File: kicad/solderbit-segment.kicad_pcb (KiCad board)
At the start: 2 copper layers, 25 x 50 mm, 15 parts, among them J1 Conn_01x05_Pin, U1 PCF8574AT, U2 PCF8574N

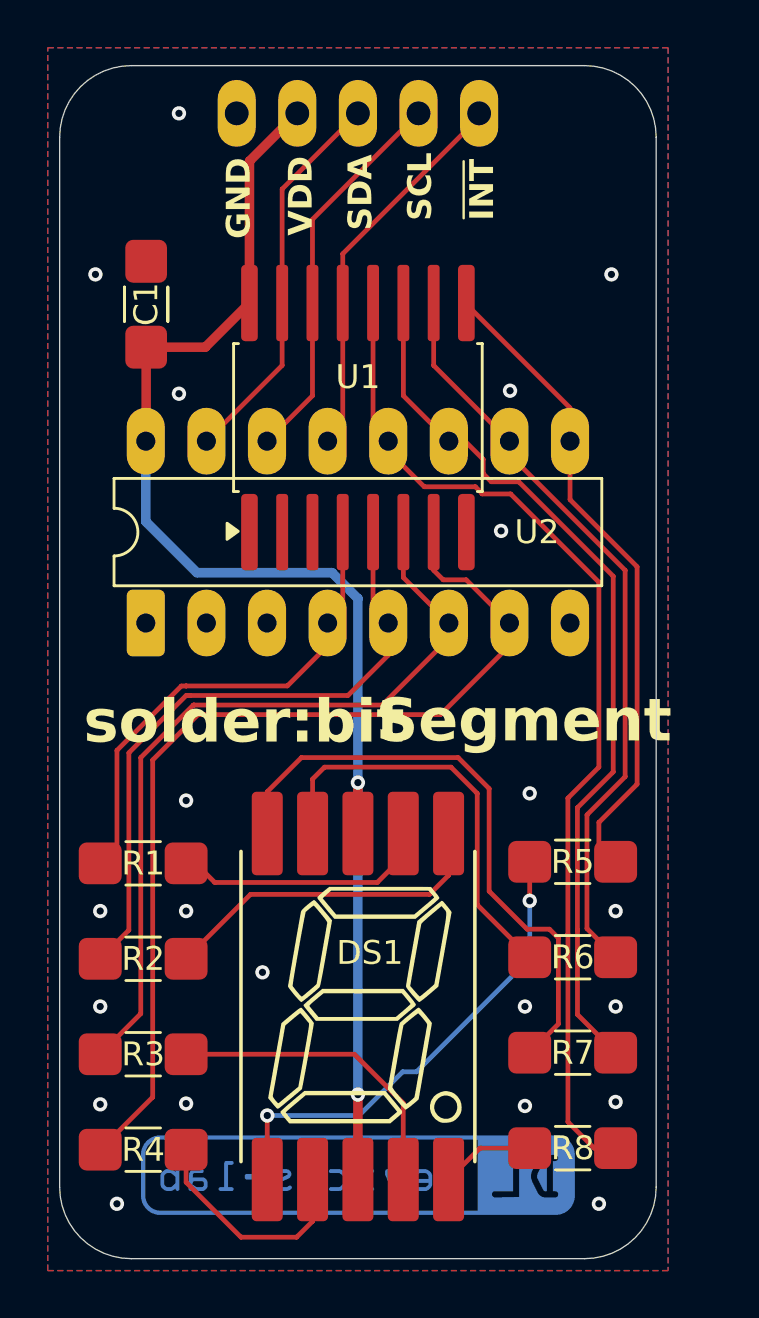
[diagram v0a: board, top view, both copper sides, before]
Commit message: Update schematic and cleanup
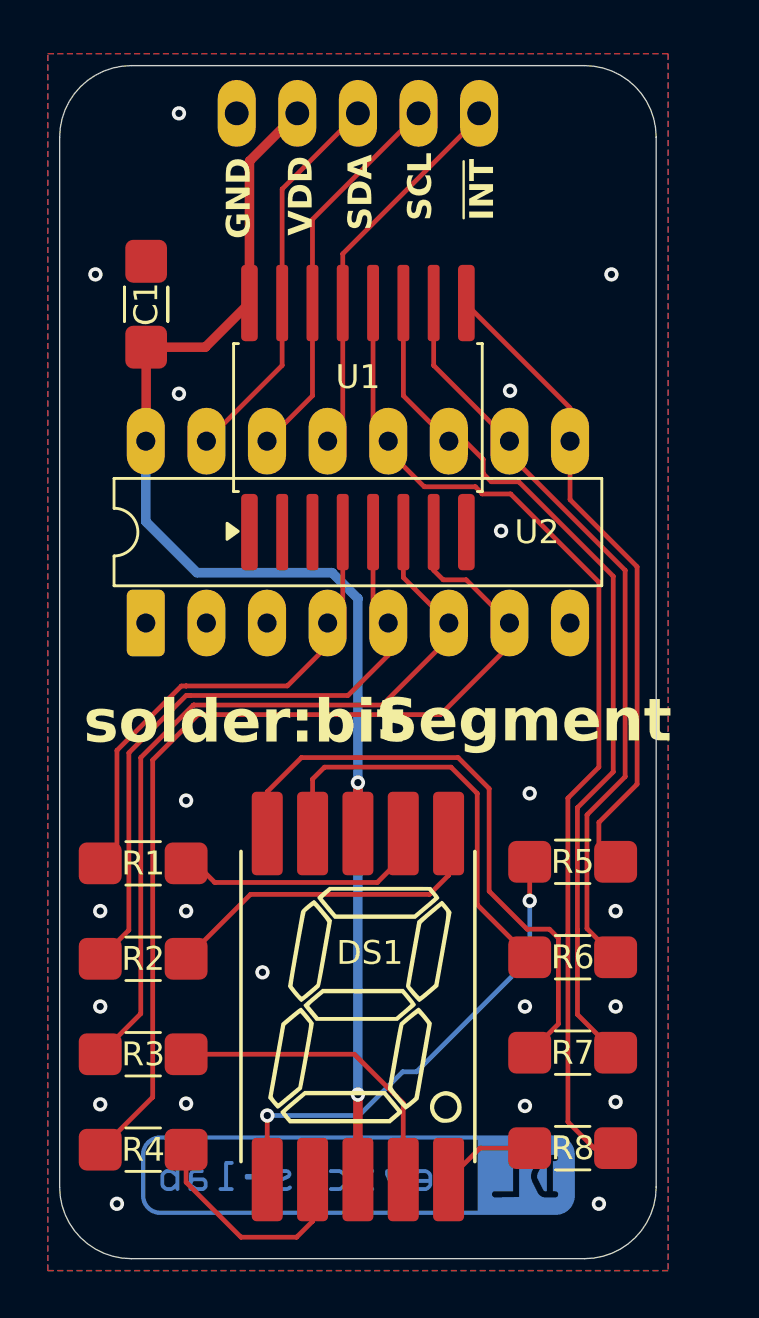
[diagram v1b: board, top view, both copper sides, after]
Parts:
- DS1: value ADMR10A0 -> ADMO10A0
- R1, R2, R3, R4, R5, R6, R7, R8: value 220R -> 150R

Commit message: Fixed the 7-segment display part number
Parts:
- DS1: value ADMO10A0 -> VDMO10A0
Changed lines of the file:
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@@
 			)
 		)
-		(property "Value" "ADMO10A0"
+		(property "Value" "VDMO10A0"
 			(at 0 -16.3 0)
 			(unlocked yes)
@@
 			)
 		)
-		(property "Onecall" "2776146"
-			(at 0 0 90)
-			(unlocked yes)
-			(layer "F.Fab")
-			(hide yes)
-			(effects
-				(font
-					(size 1 1)
-					(thickness 0.15)
-				)
-			)
-		)
 		(property "Onecall order code" "2776146"
 			(at 0 0 90)
@@
 			)
 		)
-		(property "Onecall" "3124747"
-			(at 0 0 90)
-			(unlocked yes)
-			(layer "F.Fab")
-			(hide yes)
-			(effects
-				(font
-					(size 1 1)
-					(thickness 0.15)
-				)
-			)
-		)
 		(property "Onecall order code" "3124747"
 			(at 0 0 90)
@@
 					(thickness 0.15)
 				)
-				(justify mirror)
-			)
-		)
-		(property "Onecall" "CN14490"
-			(at 0 0 270)
-			(unlocked yes)
-			(layer "B.Fab")
-			(hide yes)
-			(effects
-				(font
-					(size 1 1)
-					(thickness 0.15)
-				)

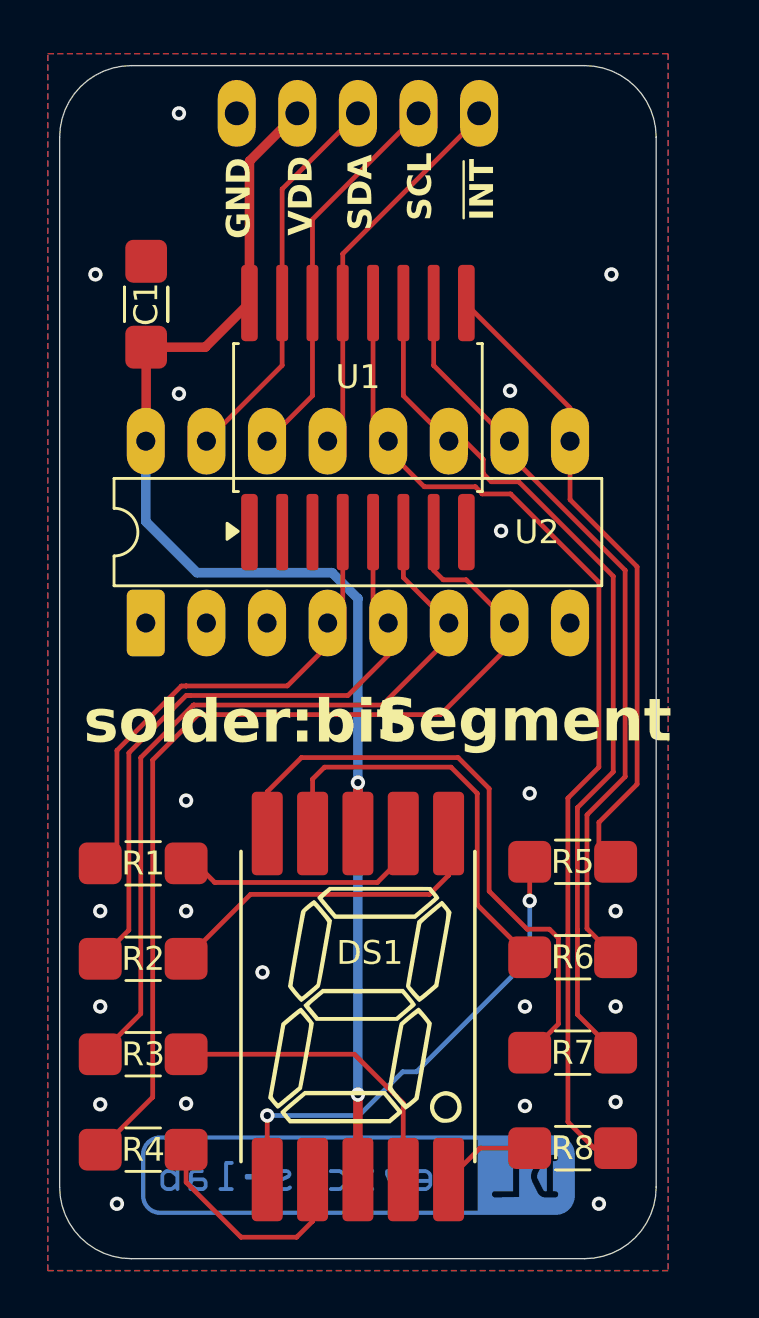
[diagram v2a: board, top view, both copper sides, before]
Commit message: New documentation
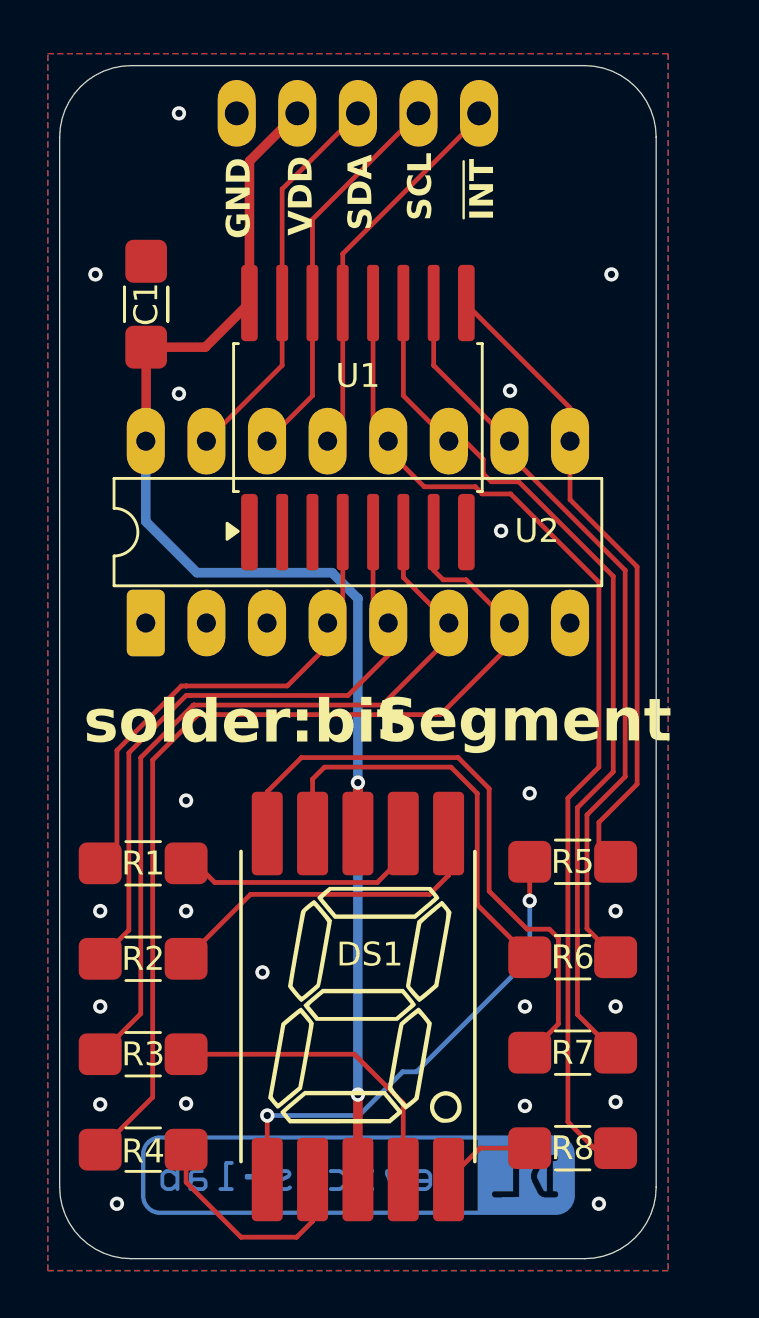
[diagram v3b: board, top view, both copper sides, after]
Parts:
- C1: footprint SolderbitSegment:C_1206 -> Solderbit_Segment:C_1206
- DS1: footprint SolderbitSegment:VDMR10 -> Solderbit_Segment:VDMR10
- J1: footprint SolderbitSegment:PinHeader_1x05_P2.54mm_Vertical -> Solderbit_Segment:PinHeader_1x05_P2.54mm_Vertical
- R1, R2, R3, R4, R5, R6, R7, R8: footprint SolderbitSegment:R_1206 -> Solderbit_Segment:R_1206
- U1: footprint SolderbitSegment:SO-16 -> Solderbit_Segment:SO-16
- U2: footprint SolderbitSegment:DIP-16 -> Solderbit_Segment:DIP-16
